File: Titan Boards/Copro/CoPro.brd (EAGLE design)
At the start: 101.6 x 101.6 mm, 83 parts, among them P2 RB1-125BAG1A, Q1 310mA/60V/1.6Ω, Q10 310mA/60V/1.6Ω, Q2 310mA/60V/1.6Ω, Q3 310mA/60V/1.6Ω, Q4 310mA/60V/1.6Ω, Q5 310mA/60V/1.6Ω, Q6 310mA/60V/1.6Ω, Q7 310mA/60V/1.6Ω, Q8 310mA/60V/1.6Ω, Q9 310mA/60V/1.6Ω, U1 SN74LVC3G04DCUT, U2 SN74LVC1G11DCKR, Y1 25Mhz, Y2 12MHz, Y3 32.768kHz

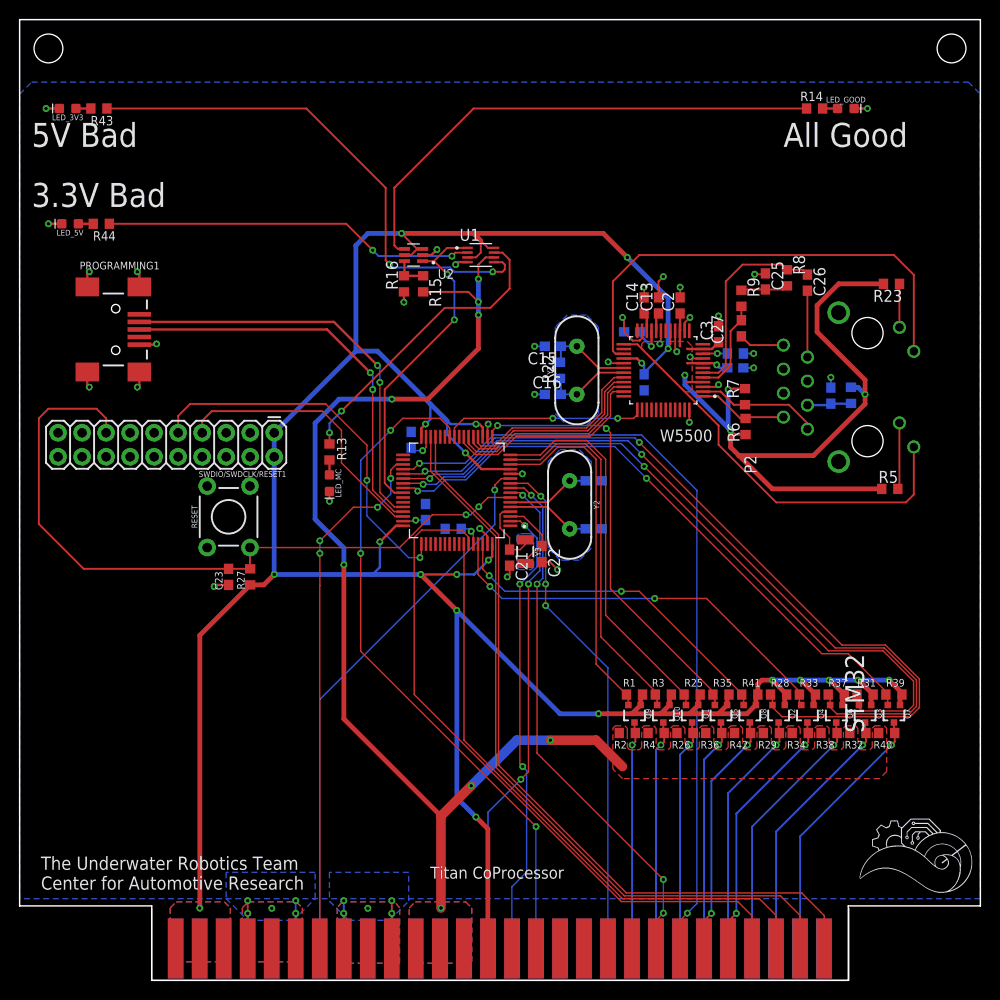
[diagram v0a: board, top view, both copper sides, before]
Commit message: Added My President Design to Board
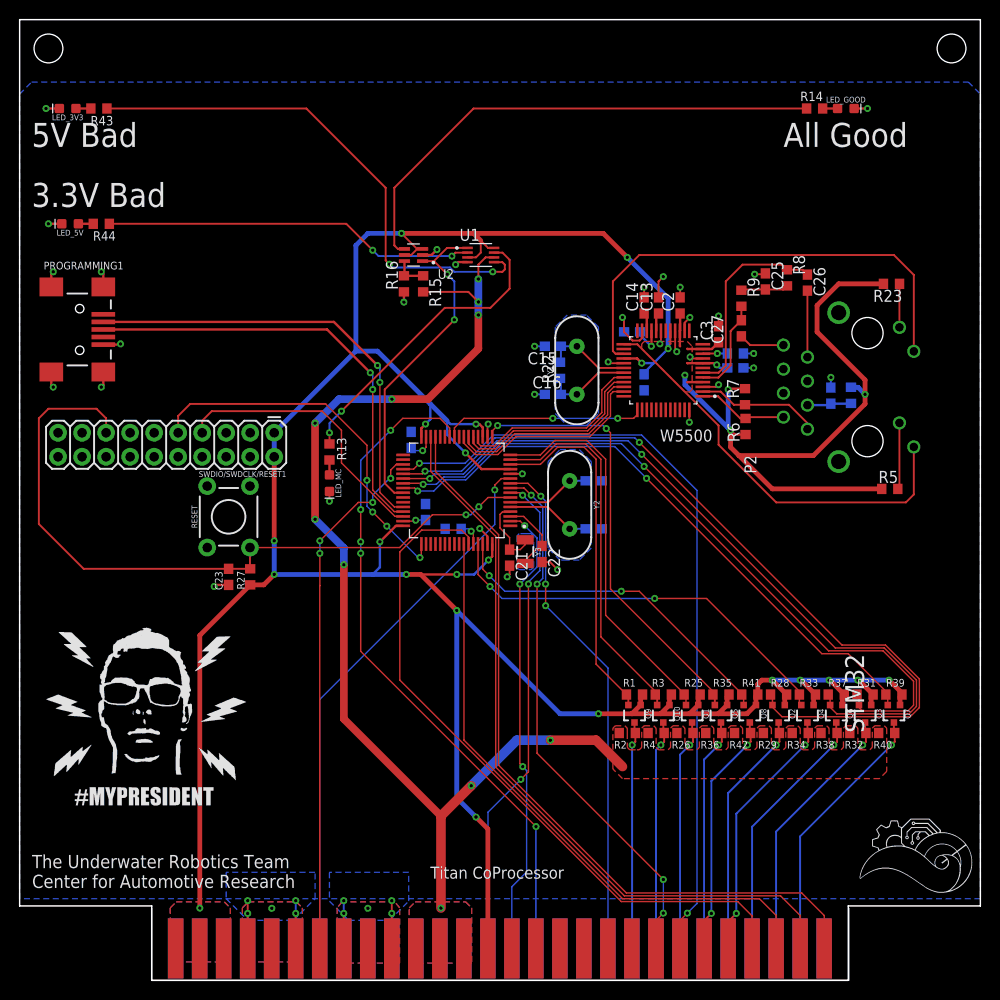
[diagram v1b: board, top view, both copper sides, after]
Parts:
- moved PROGRAMMING1 3.81 mm to (6.35, 68.8)
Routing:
- net D-: track 43.7 -> 47.5 mm
- net D+: track 43.0 -> 46.8 mm
- net +3V3: track 414.6 -> 416.1 mm, vias 27 -> 28
- net BP_SDA: track 72.6 -> 73.9 mm
- net SWCLK: track 40.5 -> 39.9 mm, vias 2 -> 4
- net SPARE_8: track 56.8 -> 56.2 mm
- net 12V_ON/OFF: vias 3 -> 5
- net +5V: vias 8 -> 10
